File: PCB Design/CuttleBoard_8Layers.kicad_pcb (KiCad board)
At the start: 8 copper layers, 50 x 50 mm, 178 parts, among them IC1 W25Q256JVEIQ TR, J1 DX07WH24JA3R1200, SW1 SW_Push, U1 LMR33630CQRNX, U15 TPS62824ADMQ, U16 ICM-20602, U19 USBLC6-2P6, U2 STM32H735VGH6, U20 ACS722xLCTR-10AB, U3 LMR33630CQRNX, U4 ICM-20602, U7 MPRLS0025PA00001A, Y1 NX2016SA

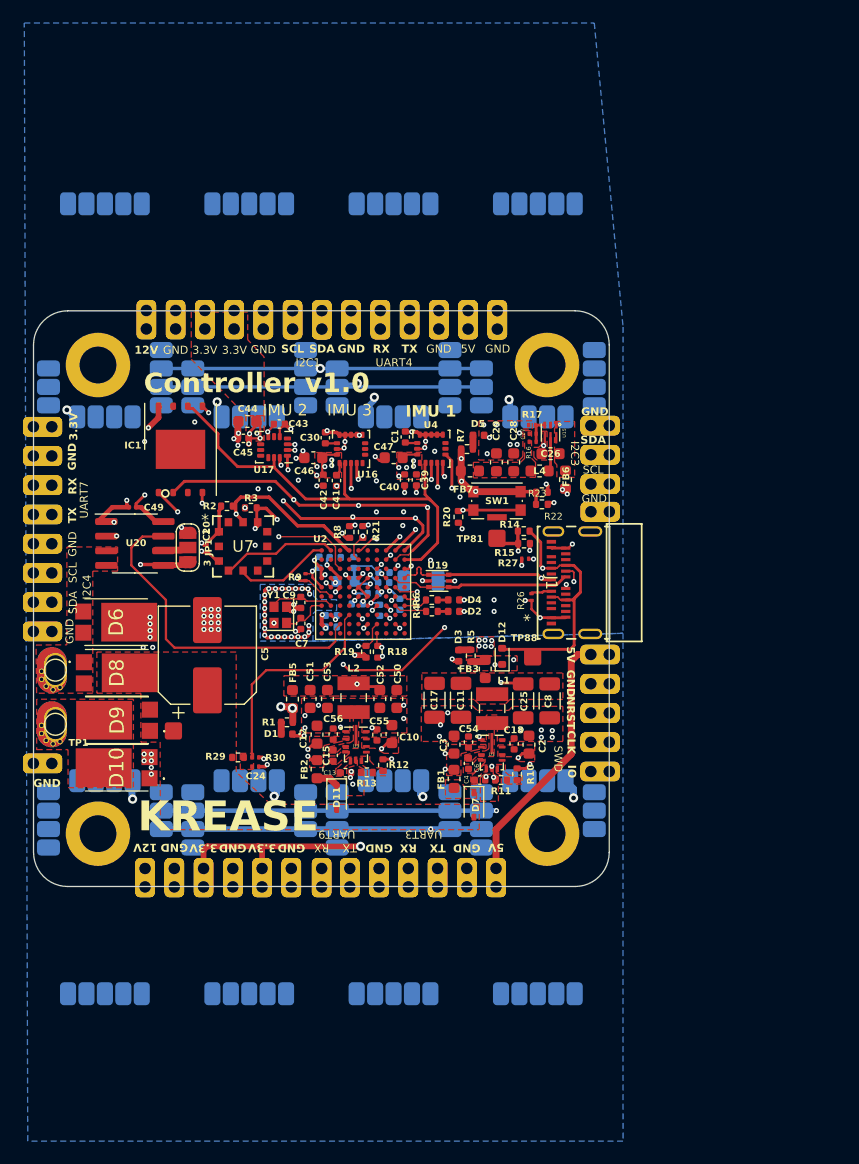
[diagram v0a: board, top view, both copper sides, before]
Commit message: readded the files after revert, sad
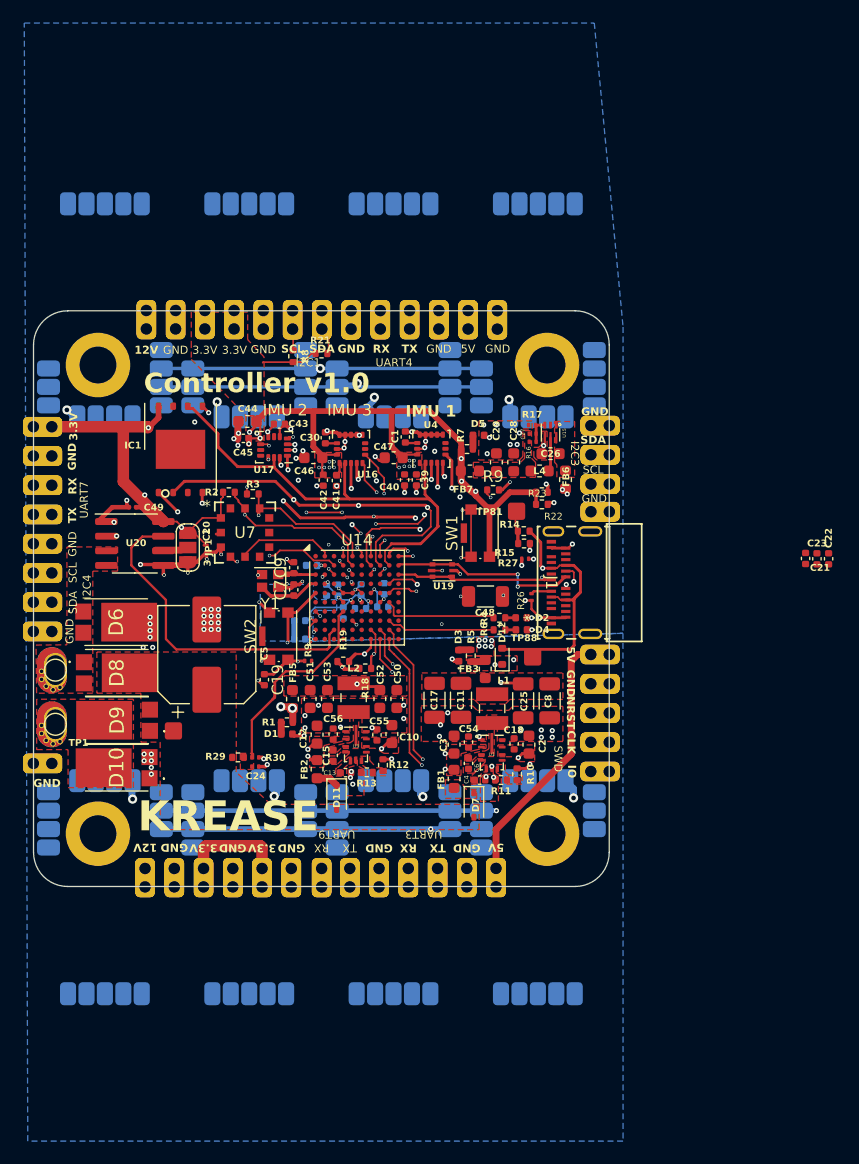
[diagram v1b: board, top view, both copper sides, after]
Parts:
- removed L3: 2.2µH, Inductor_SMD:L_0603_1608Metric
- removed R20: 2k2, Resistor_SMD:R_0402_1005Metric
- removed U2: STM32H735VGH6, Package_BGA:TFBGA-100_8x8mm_Layout10x10_P0.8mm
- added C14: 4.7µF, Capacitor_SMD:C_0402_1005Metric, B.Cu at (127.8, 99.7)
- added C16: 4.7µF, Capacitor_SMD:C_0402_1005Metric, B.Cu at (128.0, 98.1)
- added C19: 100nF, Capacitor_SMD:C_0402_1005Metric, F.Cu at (117.5, 106.0)
- added R9: 2k2, Resistor_SMD:R_0402_1005Metric, F.Cu at (137.4, 89.5)
- added SW2: SW_Push, Button_Switch_SMD:SW_Push_1P1T-SH_NO_CK_KMR2xxG, F.Cu at (118.8, 102.2)
- added U14: STM32H743VIHx, Package_BGA:TFBGA-100_8x8mm_Layout10x10_P0.8mm, F.Cu at (125.6, 98.9)
- C21, C22, C23, C48: moved to F.Cu
- moved C23 40.2 mm to (165.5, 95.5)
- moved C22 39.2 mm to (166.6, 95.5), turned to 90 degrees
- moved C21 36.6 mm to (164.6, 95.5), turned to 90 degrees
- moved R8 16.0 mm to (120.0, 77.9), turned to 90 degrees
- moved R21 15.9 mm to (122.5, 77.7), turned to 0 degrees
- moved C37 8.79 mm to (120.6, 102.5), turned to 180 degrees
- moved R9 7.28 mm to (121.3, 104.4), turned to 180 degrees
- moved C35 6.80 mm to (120.6, 100.9), turned to 180 degrees
- moved C33 6.49 mm to (123.0, 98.2)
- moved D4 6.43 mm to (139.9, 101.7)
- moved R6 6.43 mm to (138.0, 101.7)
- moved D2 5.89 mm to (139.9, 100.7)
- moved R4 5.89 mm to (138.0, 100.7)
- moved C48 5.77 mm to (136.8, 98.8)
- moved C34 5.40 mm to (125.9, 99.8), turned to 180 degrees
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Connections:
- net /PA9_USB_VBUS_sense renamed Net-(R14-Pad2)
- net /USB_D+ renamed USB_D+
- net /USB_D- renamed USB_D-
- net MISO_GYRO renamed SPI3_MISO
- net MOSI_GYRO renamed SPI3_MOSI
- net SCLK_GYRO renamed SPI3_SCK
- 3.3V pad 1: +3V3 -> +3.3V (x5)
- C20 pad 1: +3V3 -> +3.3V
- C31 pad 1: +3V3 -> +3.3V
- C32 pad 1: +3V3 -> +3.3V
- C33 pad 1: +3V3 -> +3.3V
- C34 pad 1: +3V3 -> +3.3V
- C35 pad 1: +3V3 -> +3.3V
- C36 pad 1: +3V3 -> +3.3V
- C37 pad 1: +3V3 -> +3.3V
- C38 pad 1: +3V3 -> +3.3V
- C39 pad 1: +3V3 -> +3.3V
- C40 pad 1: +3V3 -> +3.3V
- C41 pad 1: +3V3 -> +3.3V
- C42 pad 1: +3V3 -> +3.3V
- C43 pad 1: +3V3 -> +3.3V
- C44 pad 1: +3V3 -> +3.3V
- C45 pad 1: +3V3 -> +3.3V
- C46 pad 1: +3V3 -> +3.3V
- C47 pad 1: +3V3 -> +3.3V
- C49 pad 1: +3V3 -> +3.3V
- C7 pad 1: OSC_IN -> OSC_OUT
- C9 pad 1: OSC_OUT -> OSC_IN
- FB7 pad 1: +3V3 -> +3.3V
- IC1 pad 8: +3V3 -> +3.3V
- JP1 pad 1: +3V3 -> +3.3V
- R18 pad 1: +3V3 -> +3.3V
- R19 pad 1: +3V3 -> +3.3V
- R2 pad 1: +3V3 -> +3.3V
- R21 pad 1: +3V3 -> +3.3V
- R22 pad 1: +3V3 -> +3.3V
- R23 pad 1: +3V3 -> +3.3V
- R3 pad 1: +3V3 -> +3.3V
- R4 pad 1: /PC7_LED_WT -> LED_WT
- R6 pad 1: /PC8_LED_BL -> LED_BL
- R7 pad 1: +3V3 -> +3.3V
- R8 pad 1: +3V3 -> +3.3V
- RX pad 1: UART9_RX -> UART5_RX
- SW1 pad 1: Net-(U2A-BOOT0) -> BOOT0
- SW1 pad 2: +3V3 -> +3.3V
- TX pad 1: UART9_TX -> UART5_TX
- U10 pad 16: unconnected-(U10-GND-Pad16) -> GND
- U10 pad 2: unconnected-(U10-GND-Pad2) -> GND
- U10 pad 5: unconnected-(U10-GND-Pad5) -> GND
- U11 pad 16: unconnected-(U11-GND-Pad16) -> GND
- U11 pad 2: unconnected-(U11-GND-Pad2) -> GND
- U11 pad 5: unconnected-(U11-GND-Pad5) -> GND
- U12 pad 16: unconnected-(U12-GND-Pad16) -> GND
- U12 pad 2: unconnected-(U12-GND-Pad2) -> GND
- U12 pad 5: unconnected-(U12-GND-Pad5) -> GND
- U13 pad 16: unconnected-(U13-GND-Pad16) -> GND
- U13 pad 2: unconnected-(U13-GND-Pad2) -> GND
- U13 pad 5: unconnected-(U13-GND-Pad5) -> GND
- U16 pad 1: +3V3 -> +3.3V
- U16 pad 16: +3V3 -> +3.3V
- U17 pad 4: INT_IMU31 -> INT1_IMU3
- U17 pad 5: +3V3 -> +3.3V
- U17 pad 8: +3V3 -> +3.3V
- U17 pad 9: INT_IMU32 -> INT2_IMU3
- U20 pad 8: +3V3 -> +3.3V
- U4 pad 1: +3V3 -> +3.3V
- U4 pad 16: +3V3 -> +3.3V
- U5 pad 16: unconnected-(U5-GND-Pad16) -> GND
- U5 pad 2: unconnected-(U5-GND-Pad2) -> GND
- U5 pad 5: unconnected-(U5-GND-Pad5) -> GND
- U6 pad 16: unconnected-(U6-GND-Pad16) -> GND
- U6 pad 2: unconnected-(U6-GND-Pad2) -> GND
- U6 pad 5: unconnected-(U6-GND-Pad5) -> GND
- U7 pad 12: +3V3 -> +3.3V
- U8 pad 16: unconnected-(U8-GND-Pad16) -> GND
- U8 pad 2: unconnected-(U8-GND-Pad2) -> GND
- U8 pad 5: unconnected-(U8-GND-Pad5) -> GND
- U9 pad 16: unconnected-(U9-GND-Pad16) -> GND
- U9 pad 2: unconnected-(U9-GND-Pad2) -> GND
- U9 pad 5: unconnected-(U9-GND-Pad5) -> GND
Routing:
- net +3.3V: track 0.00 -> 152.9 mm, vias 0 -> 34
- net +3V3: track 94.6 -> 0.00 mm, vias 37 -> 0
- net UART9_TX: track 25.4 -> 0.00 mm, vias 1 -> 0
- net UART9_RX: track 24.8 -> 0.00 mm, vias 1 -> 0
- net UART5_TX: track 0.00 -> 24.7 mm, vias 0 -> 1
- net UART5_RX: track 0.00 -> 23.3 mm, vias 0 -> 1
- net BOOT0: track 0.00 -> 22.3 mm, vias 0 -> 4
- net UART4_RX: track 22.3 -> 0.06 mm, vias 1 -> 0
- net UART4_TX: track 20.8 -> 0.00 mm, vias 1 -> 0
- net INT1_IMU3: track 0.00 -> 17.1 mm, vias 0 -> 2
- net Net-(U2B-VFBSMPS): track 16.7 -> 0.00 mm, vias 4 -> 0
- net Net-(U2A-BOOT0): track 16.0 -> 0.00 mm, vias 2 -> 0
- net INT2_IMU3: track 0.00 -> 15.8 mm, vias 0 -> 3
- net CS_IMU3: track 0.00 -> 13.6 mm, vias 0 -> 4
- net Net-(R14-Pad2): track 15.4 -> 3.16 mm, vias 2 -> 0
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- added copper zone on F.Cu, net +3.3V
- added copper zone on In4.Cu, net +3.3V
- removed copper zone on F.Cu, net +3V3
- removed copper zone on In4.Cu, net +3V3

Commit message: Revert "STM32H743 first version"
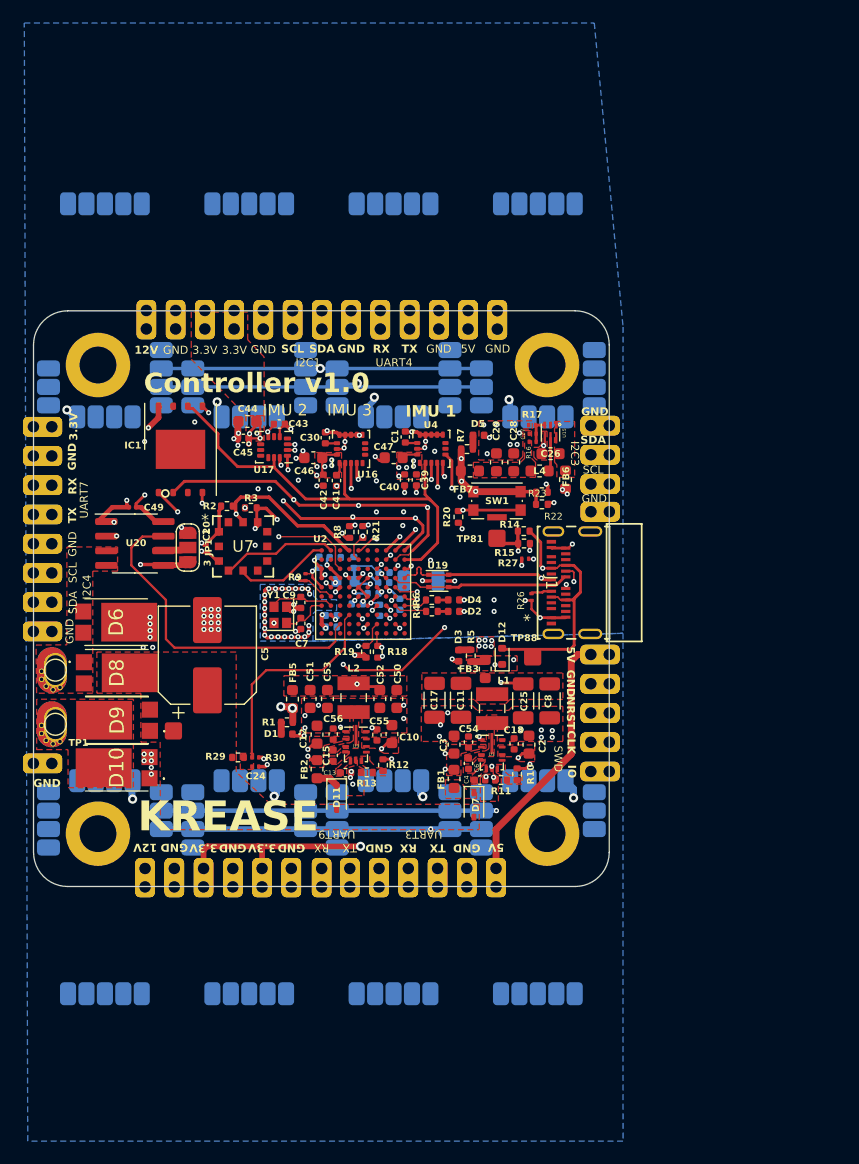
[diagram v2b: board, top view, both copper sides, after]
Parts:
- removed C14, C16: 4.7µF, Capacitor_SMD:C_0402_1005Metric
- removed C19: 100nF, Capacitor_SMD:C_0402_1005Metric
- removed the R9 at (137.4, 89.5)
- removed SW2: SW_Push, Button_Switch_SMD:SW_Push_1P1T-SH_NO_CK_KMR2xxG
- removed U14: STM32H743VIHx, Package_BGA:TFBGA-100_8x8mm_Layout10x10_P0.8mm
- added L3: 2.2µH, Inductor_SMD:L_0603_1608Metric, B.Cu at (124.6, 97.5)
- added R20: 2k2, Resistor_SMD:R_0402_1005Metric, F.Cu at (134.4, 91.9)
- added U2: STM32H735VGH6, Package_BGA:TFBGA-100_8x8mm_Layout10x10_P0.8mm, F.Cu at (126.1, 98.4)
- C21, C22, C23, C48: moved to B.Cu
- moved C23 40.2 mm to (125.3, 95.8)
- moved C22 39.2 mm to (127.6, 100.0), turned to -90 degrees
- moved C21 36.6 mm to (127.9, 96.7), turned to 0 degrees
- moved R8 16.0 mm to (125.0, 93.2), turned to -90 degrees
- moved R21 15.9 mm to (126.1, 93.2), turned to -90 degrees
- moved C37 8.79 mm to (127.9, 97.6), turned to 0 degrees
- moved R9 7.28 mm to (121.1, 97.1), turned to -90 degrees
- moved C35 6.80 mm to (127.0, 98.5), turned to 0 degrees
- moved C33 6.49 mm to (129.3, 99.5)
- moved D4 6.43 mm to (134.0, 99.1)
- moved R6 6.43 mm to (132.1, 99.1)
- moved D2 5.89 mm to (134.0, 100.1)
- moved R4 5.89 mm to (132.1, 100.1)
- moved C48 5.77 mm to (131.2, 97.4)
- moved C34 5.40 mm to (122.3, 95.8), turned to 90 degrees
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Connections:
- net Net-(R14-Pad2) renamed /PA9_USB_VBUS_sense
- net SPI3_MISO renamed MISO_GYRO
- net SPI3_MOSI renamed MOSI_GYRO
- net SPI3_SCK renamed SCLK_GYRO
- net USB_D+ renamed /USB_D+
- net USB_D- renamed /USB_D-
- 3.3V pad 1: +3.3V -> +3V3 (x5)
- C20 pad 1: +3.3V -> +3V3
- C31 pad 1: +3.3V -> +3V3
- C32 pad 1: +3.3V -> +3V3
- C33 pad 1: +3.3V -> +3V3
- C34 pad 1: +3.3V -> +3V3
- C35 pad 1: +3.3V -> +3V3
- C36 pad 1: +3.3V -> +3V3
- C37 pad 1: +3.3V -> +3V3
- C38 pad 1: +3.3V -> +3V3
- C39 pad 1: +3.3V -> +3V3
- C40 pad 1: +3.3V -> +3V3
- C41 pad 1: +3.3V -> +3V3
- C42 pad 1: +3.3V -> +3V3
- C43 pad 1: +3.3V -> +3V3
- C44 pad 1: +3.3V -> +3V3
- C45 pad 1: +3.3V -> +3V3
- C46 pad 1: +3.3V -> +3V3
- C47 pad 1: +3.3V -> +3V3
- C49 pad 1: +3.3V -> +3V3
- C7 pad 1: OSC_OUT -> OSC_IN
- C9 pad 1: OSC_IN -> OSC_OUT
- FB7 pad 1: +3.3V -> +3V3
- IC1 pad 8: +3.3V -> +3V3
- JP1 pad 1: +3.3V -> +3V3
- R18 pad 1: +3.3V -> +3V3
- R19 pad 1: +3.3V -> +3V3
- R2 pad 1: +3.3V -> +3V3
- R21 pad 1: +3.3V -> +3V3
- R22 pad 1: +3.3V -> +3V3
- R23 pad 1: +3.3V -> +3V3
- R3 pad 1: +3.3V -> +3V3
- R4 pad 1: LED_WT -> /PC7_LED_WT
- R6 pad 1: LED_BL -> /PC8_LED_BL
- R7 pad 1: +3.3V -> +3V3
- R8 pad 1: +3.3V -> +3V3
- RX pad 1: UART5_RX -> UART9_RX
- SW1 pad 1: BOOT0 -> Net-(U2A-BOOT0)
- SW1 pad 2: +3.3V -> +3V3
- TX pad 1: UART5_TX -> UART9_TX
- U10 pad 16: GND -> unconnected-(U10-GND-Pad16)
- U10 pad 2: GND -> unconnected-(U10-GND-Pad2)
- U10 pad 5: GND -> unconnected-(U10-GND-Pad5)
- U11 pad 16: GND -> unconnected-(U11-GND-Pad16)
- U11 pad 2: GND -> unconnected-(U11-GND-Pad2)
- U11 pad 5: GND -> unconnected-(U11-GND-Pad5)
- U12 pad 16: GND -> unconnected-(U12-GND-Pad16)
- U12 pad 2: GND -> unconnected-(U12-GND-Pad2)
- U12 pad 5: GND -> unconnected-(U12-GND-Pad5)
- U13 pad 16: GND -> unconnected-(U13-GND-Pad16)
- U13 pad 2: GND -> unconnected-(U13-GND-Pad2)
- U13 pad 5: GND -> unconnected-(U13-GND-Pad5)
- U16 pad 1: +3.3V -> +3V3
- U16 pad 16: +3.3V -> +3V3
- U17 pad 4: INT1_IMU3 -> INT_IMU31
- U17 pad 5: +3.3V -> +3V3
- U17 pad 8: +3.3V -> +3V3
- U17 pad 9: INT2_IMU3 -> INT_IMU32
- U20 pad 8: +3.3V -> +3V3
- U4 pad 1: +3.3V -> +3V3
- U4 pad 16: +3.3V -> +3V3
- U5 pad 16: GND -> unconnected-(U5-GND-Pad16)
- U5 pad 2: GND -> unconnected-(U5-GND-Pad2)
- U5 pad 5: GND -> unconnected-(U5-GND-Pad5)
- U6 pad 16: GND -> unconnected-(U6-GND-Pad16)
- U6 pad 2: GND -> unconnected-(U6-GND-Pad2)
- U6 pad 5: GND -> unconnected-(U6-GND-Pad5)
- U7 pad 12: +3.3V -> +3V3
- U8 pad 16: GND -> unconnected-(U8-GND-Pad16)
- U8 pad 2: GND -> unconnected-(U8-GND-Pad2)
- U8 pad 5: GND -> unconnected-(U8-GND-Pad5)
- U9 pad 16: GND -> unconnected-(U9-GND-Pad16)
- U9 pad 2: GND -> unconnected-(U9-GND-Pad2)
- U9 pad 5: GND -> unconnected-(U9-GND-Pad5)
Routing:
- net +3.3V: track 152.9 -> 0.00 mm, vias 34 -> 0
- net +3V3: track 0.00 -> 94.6 mm, vias 0 -> 37
- net UART9_TX: track 0.00 -> 25.4 mm, vias 0 -> 1
- net UART9_RX: track 0.00 -> 24.8 mm, vias 0 -> 1
- net UART5_TX: track 24.7 -> 0.00 mm, vias 1 -> 0
- net UART5_RX: track 23.3 -> 0.00 mm, vias 1 -> 0
- net BOOT0: track 22.3 -> 0.00 mm, vias 4 -> 0
- net UART4_RX: track 0.06 -> 22.3 mm, vias 0 -> 1
- net UART4_TX: track 0.00 -> 20.8 mm, vias 0 -> 1
- net INT1_IMU3: track 17.1 -> 0.00 mm, vias 2 -> 0
- net Net-(U2B-VFBSMPS): track 0.00 -> 16.7 mm, vias 0 -> 4
- net Net-(U2A-BOOT0): track 0.00 -> 16.0 mm, vias 0 -> 2
- net INT2_IMU3: track 15.8 -> 0.00 mm, vias 3 -> 0
- net CS_IMU3: track 13.6 -> 0.00 mm, vias 4 -> 0
- net /PA9_USB_VBUS_sense: track 3.16 -> 15.4 mm, vias 0 -> 2
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- added copper zone on F.Cu, net +3V3
- added copper zone on In4.Cu, net +3V3
- removed copper zone on F.Cu, net +3.3V
- removed copper zone on In4.Cu, net +3.3V
